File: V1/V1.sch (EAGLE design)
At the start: 72 parts, among them Q1 MOSFET-NCHANNEL2N7002PW, Q2 MOSFET-NCHANNEL2N7002PW, U1 MCP2510SO, U2 MCP2561, U3 ATMEGA328P_TQFP, Y1 16MHz

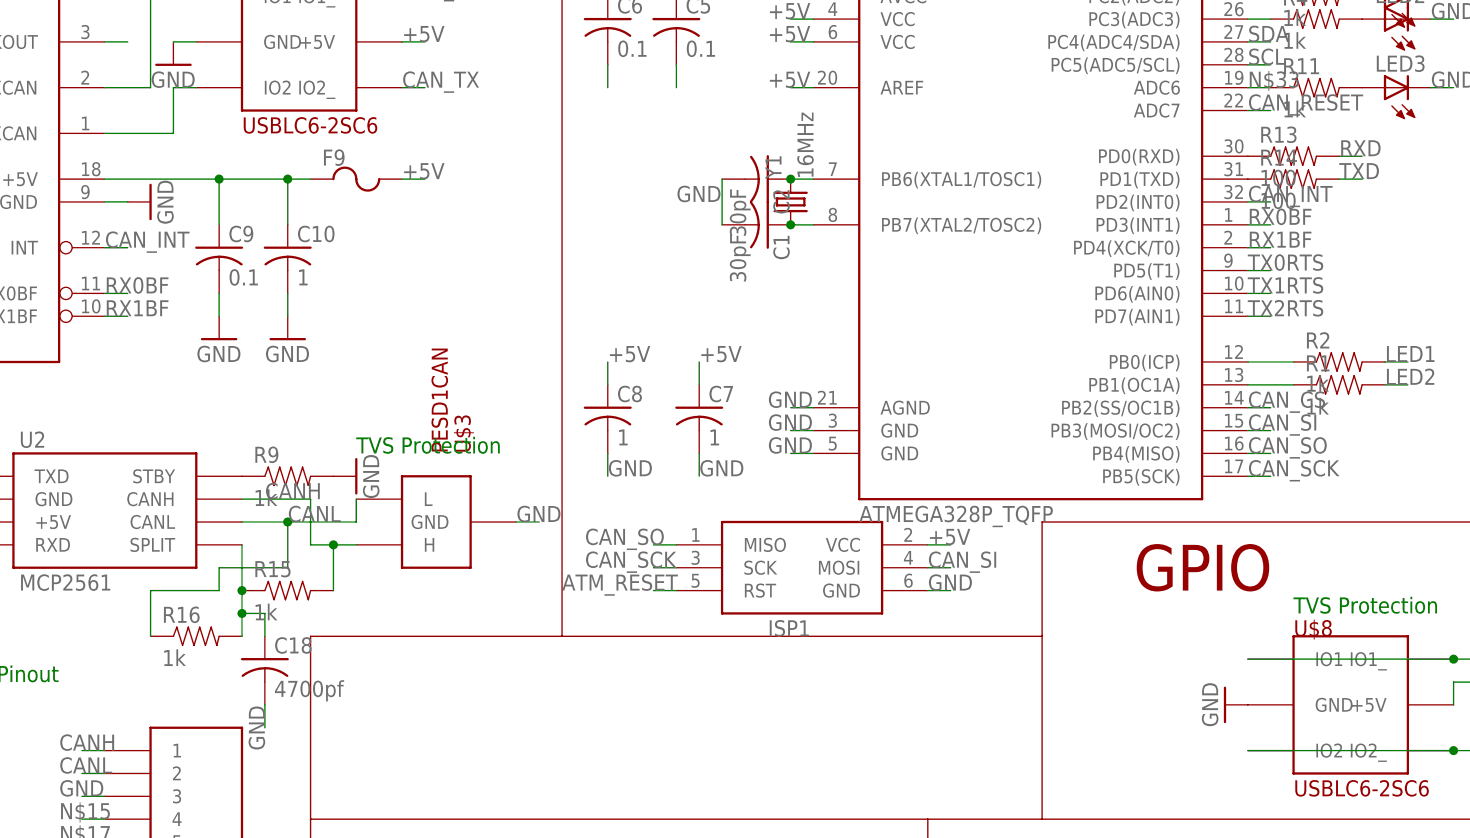
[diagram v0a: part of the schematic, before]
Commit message: update
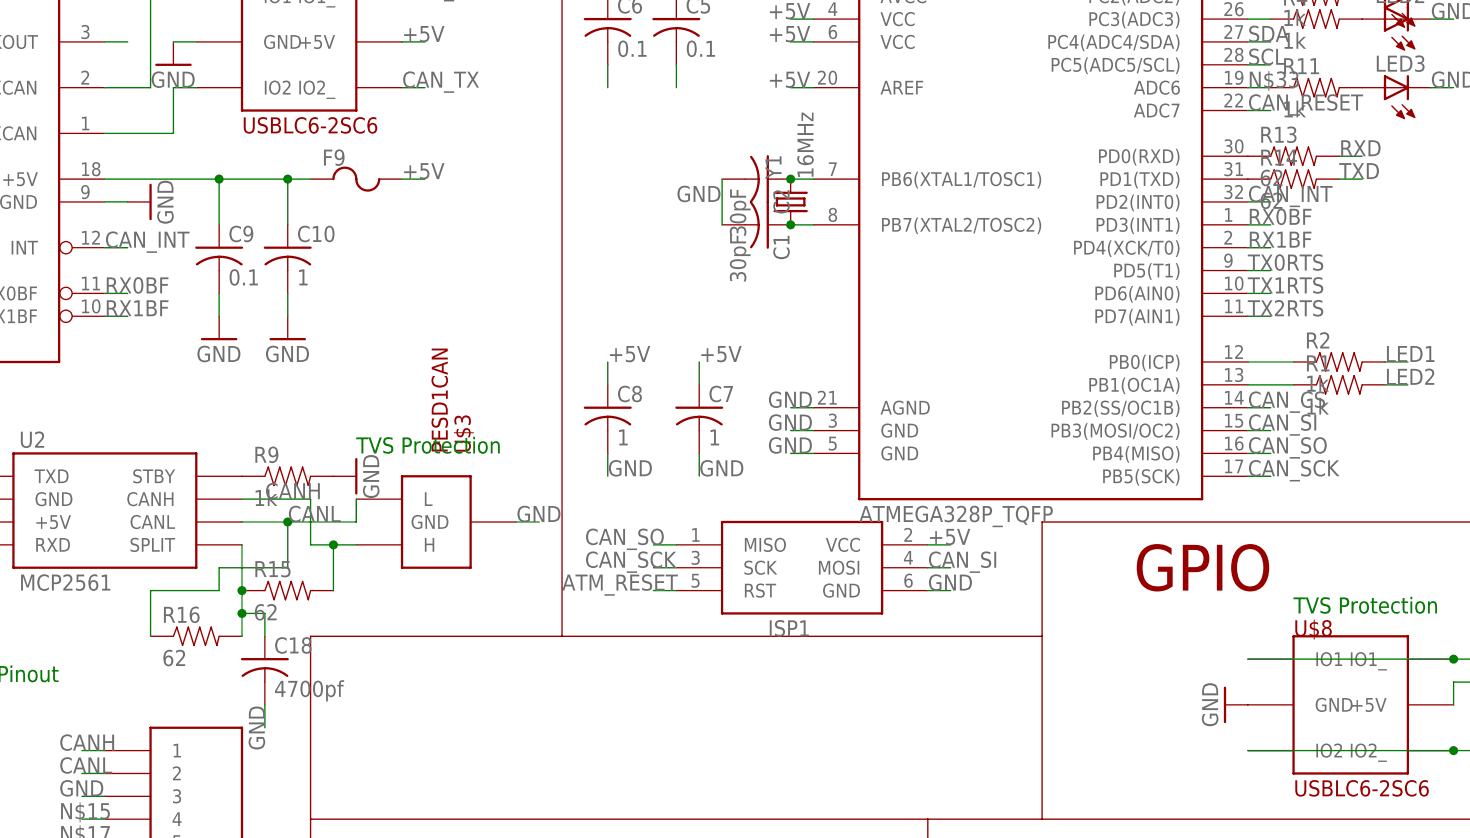
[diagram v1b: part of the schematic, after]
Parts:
- R13, R14: value 100 -> 62
- R15, R16: value 1k -> 62
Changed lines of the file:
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@@
 <?xml version="1.0" encoding="utf-8"?>
 <!DOCTYPE eagle SYSTEM "eagle.dtd">
-<eagle version="7.6.0">
+<eagle version="7.4.0">
 <drawing>
 <settings>
@@
 <part name="R11" library="SparkFun-Resistors" deviceset="RESISTOR" device="0603-RES" value="1k"/>
 <part name="R12" library="SparkFun-Resistors" deviceset="RESISTOR" device="0603-RES" value="10k"/>
-<part name="R13" library="SparkFun-Resistors" deviceset="RESISTOR" device="0603-RES" value="100"/>
-<part name="R14" library="SparkFun-Resistors" deviceset="RESISTOR" device="0603-RES" value="100"/>
+<part name="R13" library="SparkFun-Resistors" deviceset="RESISTOR" device="0603-RES" value="62"/>
+<part name="R14" library="SparkFun-Resistors" deviceset="RESISTOR" device="0603-RES" value="62"/>
 <part name="U$9" library="USBLC6-2SC6" deviceset="USBLC6-2SC6" device=""/>
 <part name="F13" library="polyfuse" deviceset="POLYFUSE" device=""/>
@@
 <part name="GND16" library="E-P-008-R1.2" deviceset="GND" device=""/>
 <part name="GND17" library="E-P-008-R1.2" deviceset="GND" device=""/>
-<part name="R15" library="SparkFun-Resistors" deviceset="RESISTOR" device="0603-RES" value="1k"/>
-<part name="R16" library="SparkFun-Resistors" deviceset="RESISTOR" device="0603-RES" value="1k"/>
+<part name="R15" library="SparkFun-Resistors" deviceset="RESISTOR" device="0603-RES" value="62"/>
+<part name="R16" library="SparkFun-Resistors" deviceset="RESISTOR" device="0603-RES" value="62"/>
 <part name="C18" library="adafruit" deviceset="C-US" device="C0603K" value="4700pf"/>
 </parts>
